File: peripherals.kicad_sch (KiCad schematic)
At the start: 18 parts, among them IC5 ${ALTIUM_VALUE}, IC6 ${ALTIUM_VALUE}, IC7 ${ALTIUM_VALUE}, J7 *

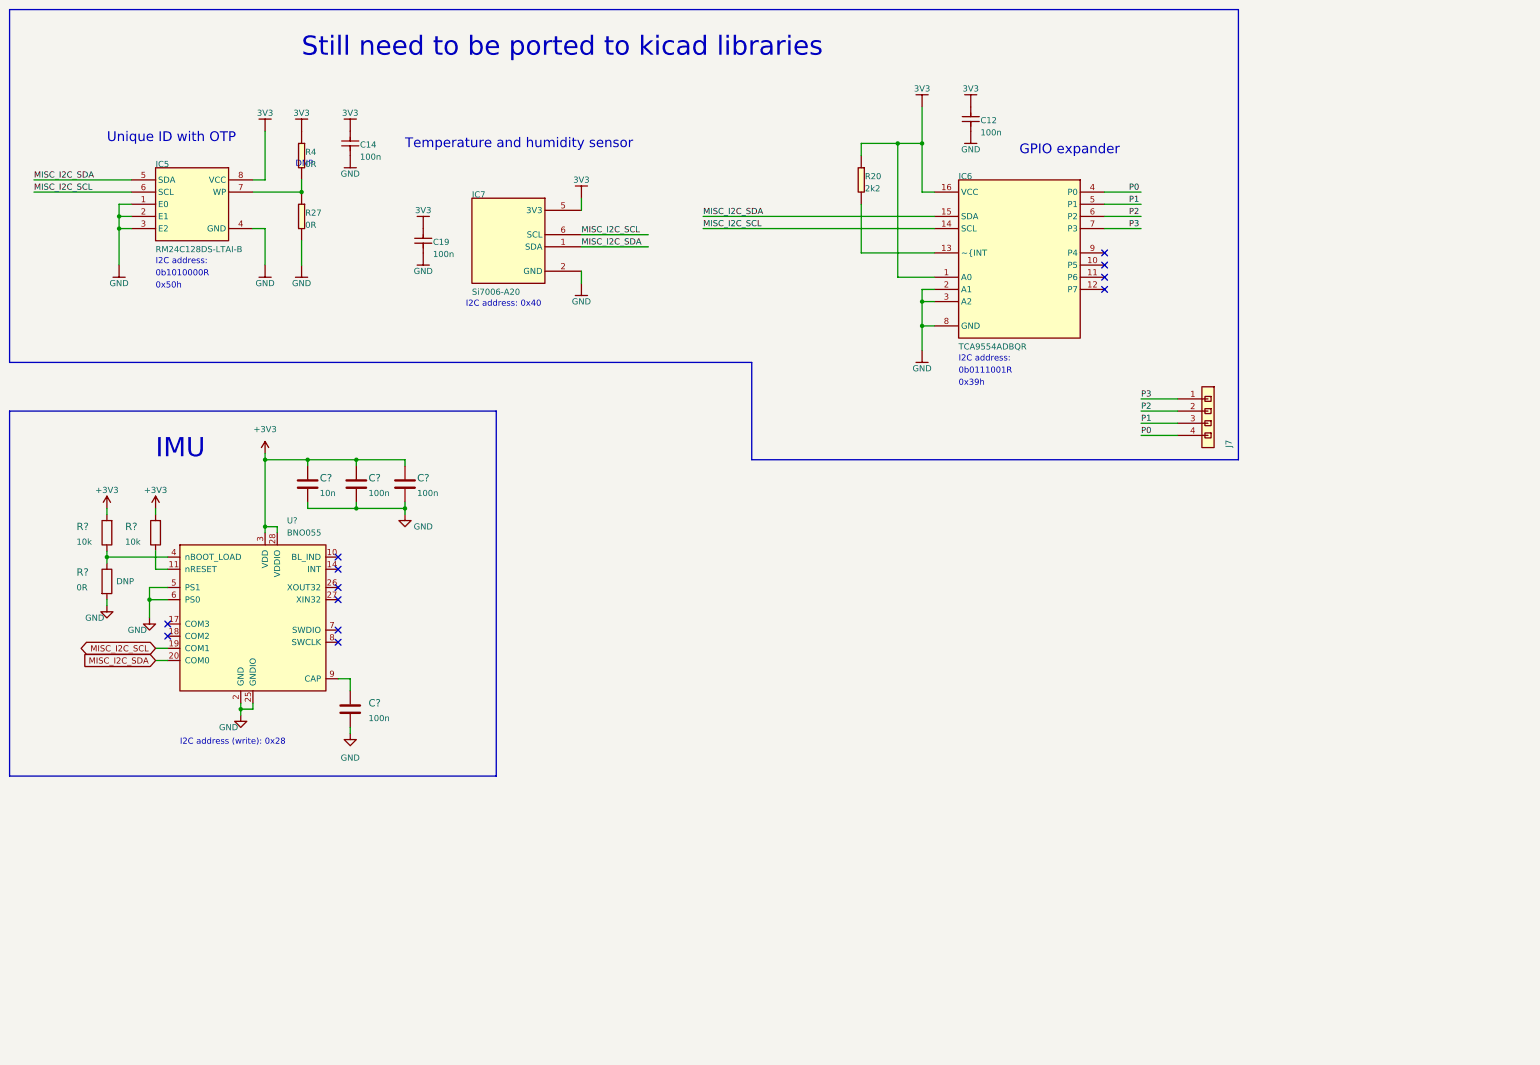
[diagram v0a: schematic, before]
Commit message: Fixes suggested in review
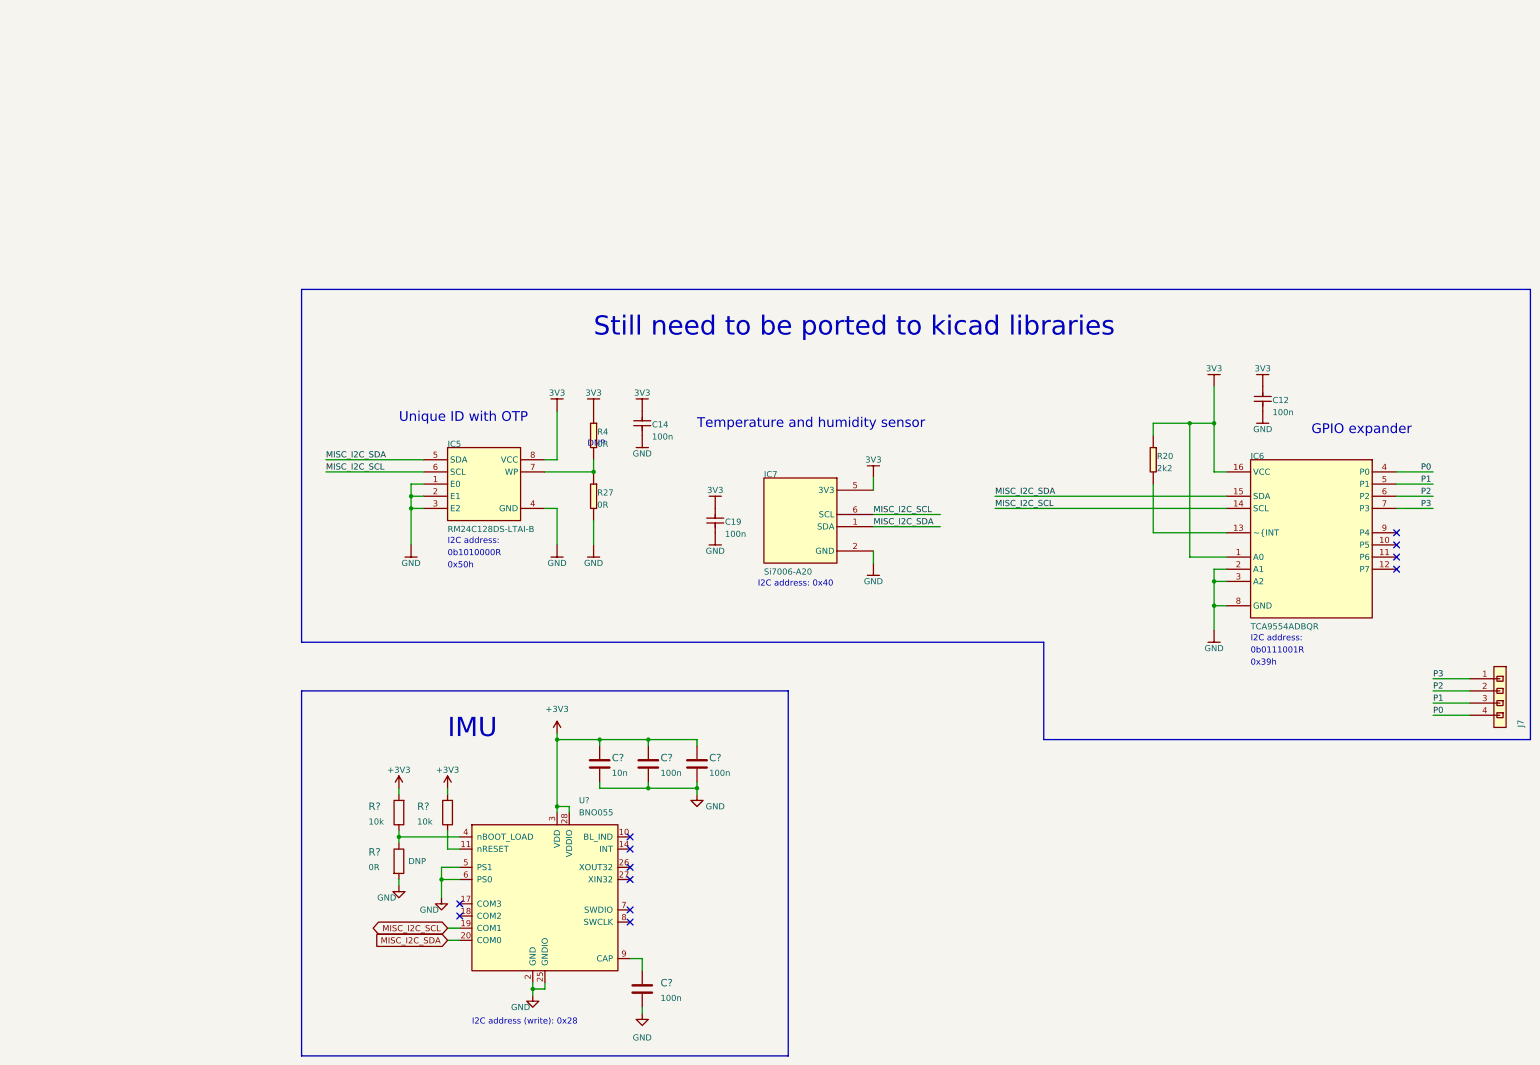
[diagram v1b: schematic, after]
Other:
- moved on the sheet: C12, C14, C19, C?, IC5, IC6, IC7, J7, R20, R27, R4, R?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
